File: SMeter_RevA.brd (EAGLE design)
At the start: 49 x 29 mm, 46 parts, among them IC1 AD8307, IC2 AD603, IC3 TL081

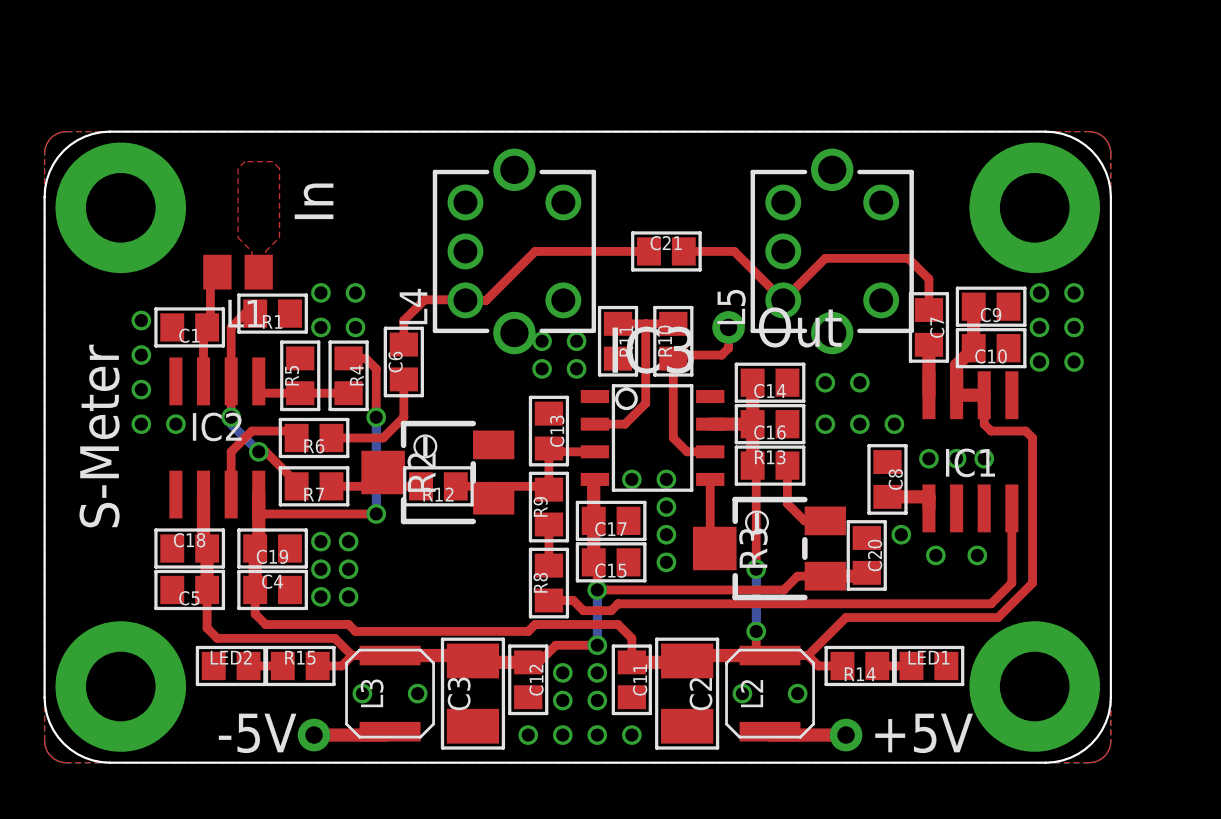
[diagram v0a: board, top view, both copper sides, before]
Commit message: Revision B finalized
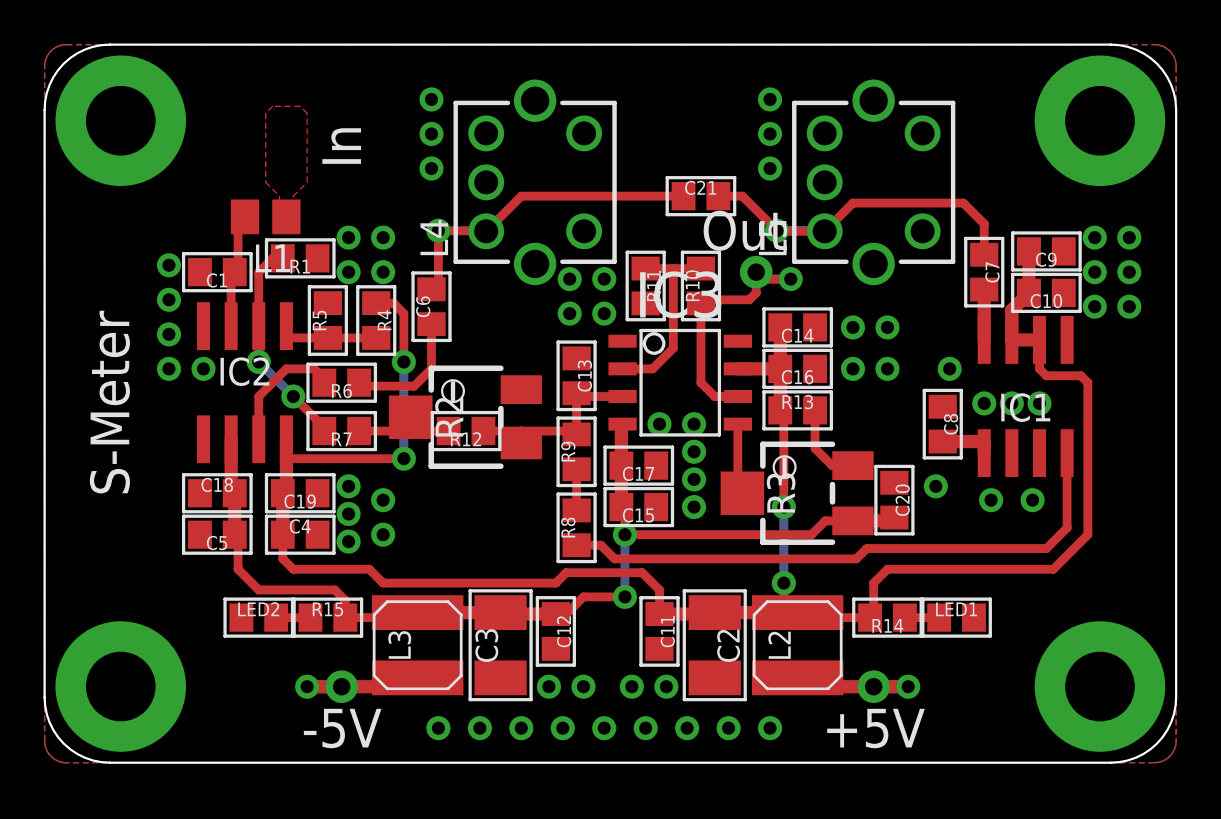
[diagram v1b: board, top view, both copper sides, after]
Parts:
- C2, C3: value 33u -> 47u
- L2, L3: value (none) -> 100uH
- moved L5 3.70 mm to (38.1, 26.7)
- moved C9 3.59 mm to (46.0, 23.5)
- moved IC1 3.59 mm to (45.1, 16.8)
- moved C10 3.59 mm to (46.0, 21.6)
- moved C7 3.59 mm to (43.2, 22.5)
- moved C8 3.59 mm to (41.3, 15.6)
- moved L4 3.31 mm to (22.5, 26.7)
- moved C21 3.00 mm to (30.2, 26.0)
- moved C14 2.84 mm to (34.6, 20.0)
- moved C13 2.84 mm to (24.4, 17.8)
- moved C16 2.84 mm to (34.6, 18.1)
- moved R3 2.84 mm to (34.6, 12.4)
- moved C19 2.84 mm to (11.7, 12.4)
- moved C15 2.84 mm to (27.3, 11.7)
- moved C18 2.84 mm to (7.94, 12.4)
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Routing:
- net OUT: track 9.30 -> 12.7 mm, vias 1 -> 2
- net +5V_IN: track 3.65 -> 7.07 mm, vias 1 -> 2
- net -5V_IN: track 3.56 -> 6.95 mm, vias 1 -> 2
- net N$11: track 13.7 -> 17.0 mm, vias 0 -> 1
- net N$20: track 14.8 -> 17.5 mm, vias 0 -> 1
- net +5V: track 90.8 -> 92.4 mm
- net N$14: track 25.4 -> 26.8 mm
- net -5V: track 47.5 -> 46.8 mm
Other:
- board size 49 x 29 mm -> 52 x 33 mm
